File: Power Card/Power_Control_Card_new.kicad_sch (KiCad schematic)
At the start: 20 parts, among them J4 Conn_01x04_Pin, Q1 IRF5305PbF, Q2 IRF5305PbF, U3 TSR2-2450, U4 TSR2-2433, U5 MCP9808_MSOP

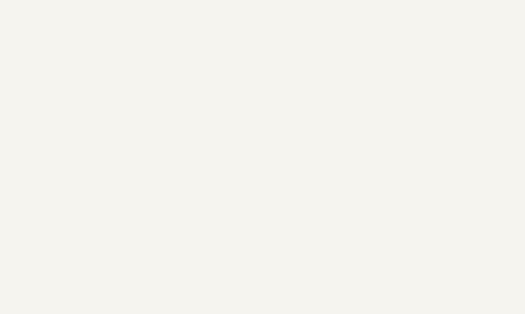
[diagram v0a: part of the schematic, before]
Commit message: testing
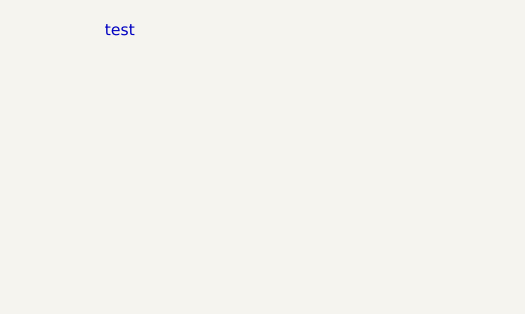
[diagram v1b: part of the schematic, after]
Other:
- note added: "test"
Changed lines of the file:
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@@
+		)
+	)
+	(text "test\n"
+		(exclude_from_sim no)
+		(at 33.528 23.114 0)
+		(effects
+			(font
+				(size 1.27 1.27)
+			)
 		)
 	)

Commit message: testing
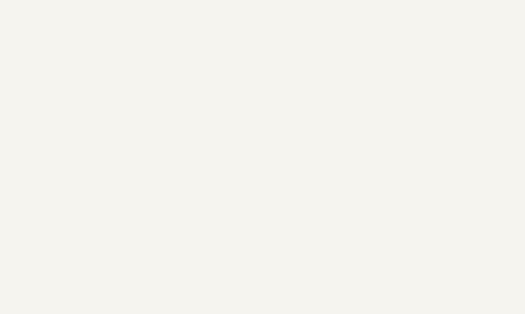
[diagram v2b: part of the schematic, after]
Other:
- note removed: "test"
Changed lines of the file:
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@@
-		)
-	)
-	(text "test\n"
-		(exclude_from_sim no)
-		(at 33.528 23.114 0)
-		(effects
-			(font
-				(size 1.27 1.27)
-			)
 		)
 	)
